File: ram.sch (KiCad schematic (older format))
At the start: 7 parts, among them U1 LFE5U-85F-6BG381C

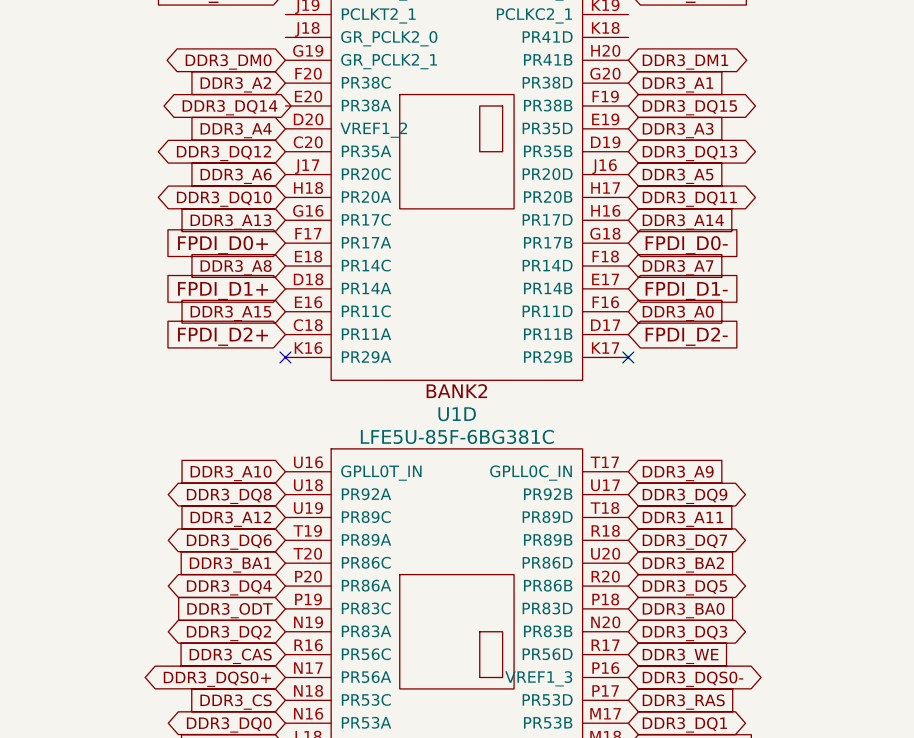
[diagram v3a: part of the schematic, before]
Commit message: More DDR3 routing
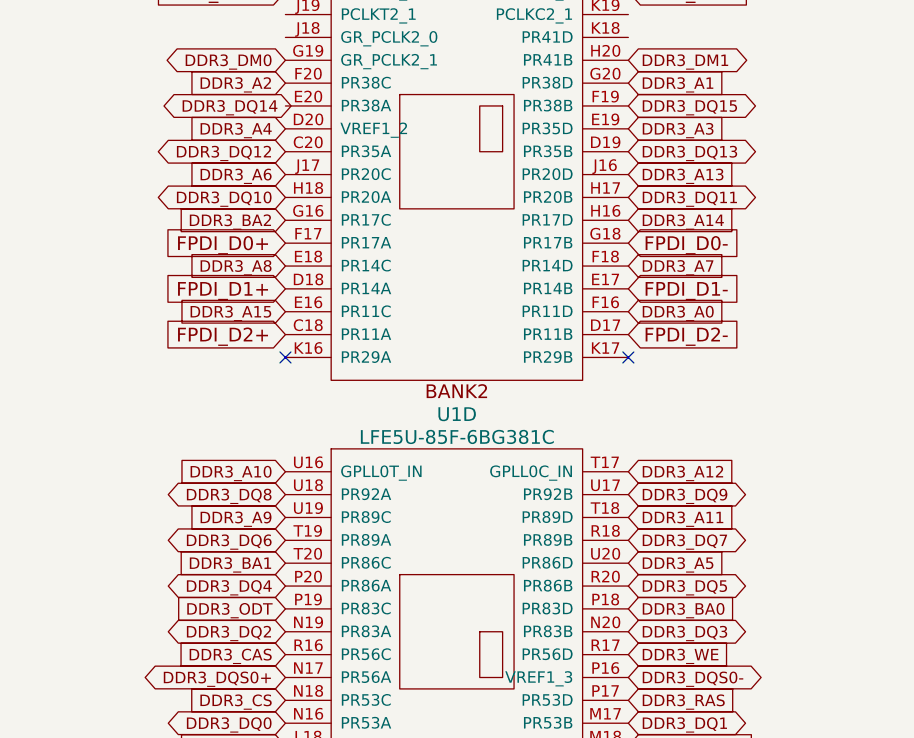
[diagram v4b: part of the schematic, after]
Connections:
- net DDR3_A12: now also U1.T17 (GPLL0C_IN); no longer U1.U19 (PR89C)
- net DDR3_A13: now also U1.J16 (PR20D); no longer U1.G16 (PR17C)
- net DDR3_A5: now also U1.U20 (PR86D); no longer U1.J16 (PR20D)
- net DDR3_A9: now also U1.U19 (PR89C); no longer U1.T17 (GPLL0C_IN)
- net DDR3_BA2: now also U1.G16 (PR17C); no longer U1.U20 (PR86D)
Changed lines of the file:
@@
 Text GLabel 6600 2300 0    50   Input ~ 0
 DDR3_A4
-Text GLabel 8100 2500 2    50   Input ~ 0
+Text GLabel 8100 4200 2    50   Input ~ 0
 DDR3_A5
 Text GLabel 6600 2500 0    50   Input ~ 0
@@
 Text GLabel 6600 2900 0    50   Input ~ 0
 DDR3_A8
-Text GLabel 8100 3800 2    50   Input ~ 0
+Text GLabel 6600 4000 0    50   Input ~ 0
 DDR3_A9
 Text GLabel 6600 3800 0    50   Input ~ 0
@@
 Text GLabel 8100 4000 2    50   Input ~ 0
 DDR3_A11
-Text GLabel 6600 4000 0    50   Input ~ 0
+Text GLabel 8100 3800 2    50   Input ~ 0
 DDR3_A12
-Text GLabel 6600 2700 0    50   Input ~ 0
+Text GLabel 8100 2500 2    50   Input ~ 0
 DDR3_A13
 Text GLabel 8100 2700 2    50   Input ~ 0
@@
 Text GLabel 6600 4200 0    50   Input ~ 0
 DDR3_BA1
-Text GLabel 8100 4200 2    50   Input ~ 0
+Text GLabel 6600 2700 0    50   Input ~ 0
 DDR3_BA2
 Text GLabel 6600 5300 0    50   Input ~ 0

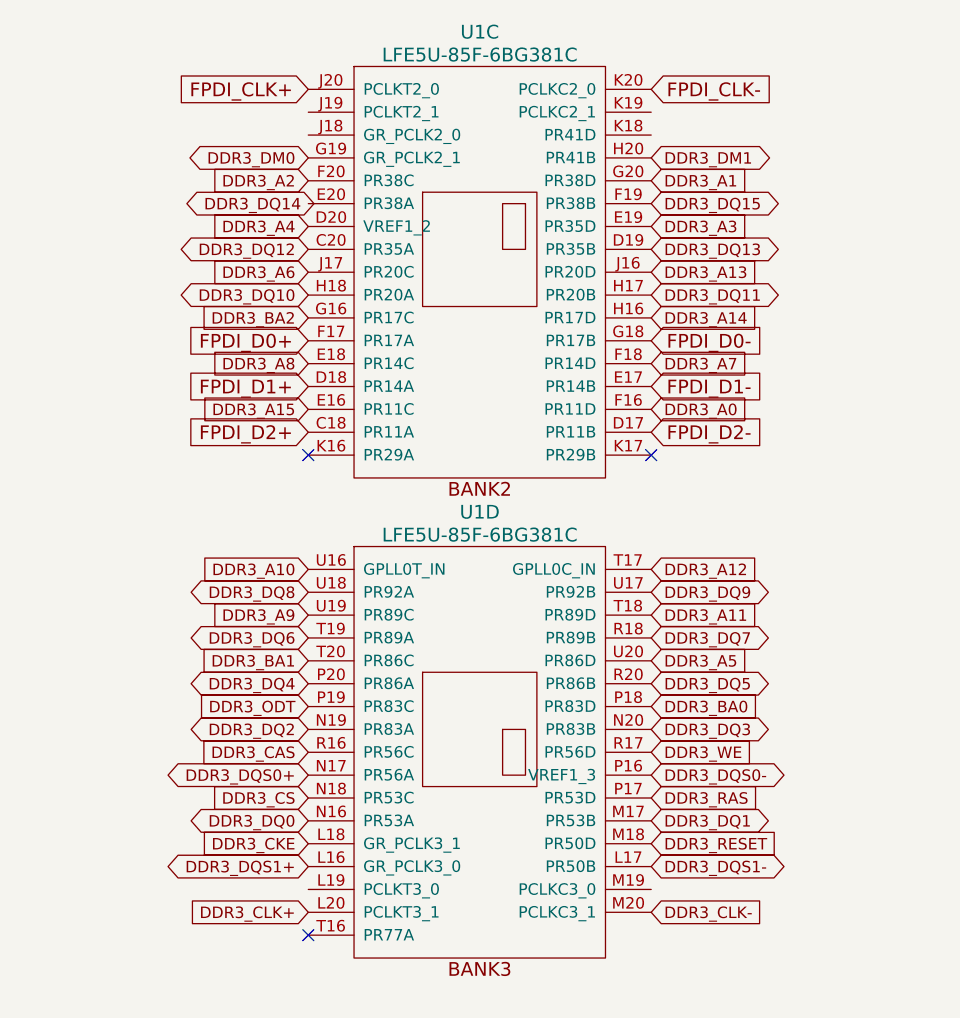
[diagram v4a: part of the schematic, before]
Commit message: Initial DDR3 signals routing
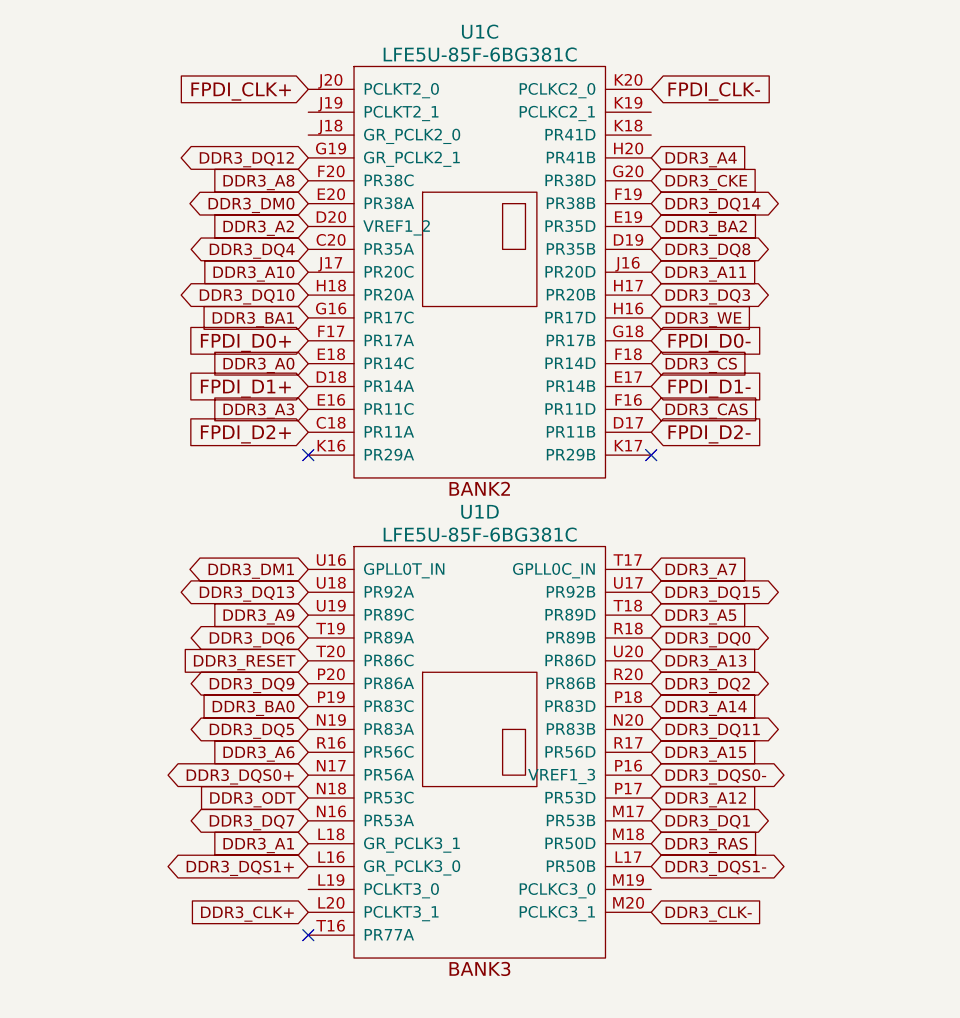
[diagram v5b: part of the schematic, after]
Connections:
- net DDR3_A0: now also U1.E18 (PR14C); no longer U1.F16 (PR11D)
- net DDR3_A1: now also U1.L18 (GR_PCLK3_1); no longer U1.G20 (PR38D)
- net DDR3_A10: now also U1.J17 (PR20C); no longer U1.U16 (GPLL0T_IN)
- net DDR3_A11: now also U1.J16 (PR20D); no longer U1.T18 (PR89D)
- net DDR3_A12: now also U1.P17 (PR53D); no longer U1.T17 (GPLL0C_IN)
- net DDR3_A13: now also U1.U20 (PR86D); no longer U1.J16 (PR20D)
- net DDR3_A14: now also U1.P18 (PR83D); no longer U1.H16 (PR17D)
- net DDR3_A15: now also U1.R17 (PR56D); no longer U1.E16 (PR11C)
- net DDR3_A2: now also U1.D20 (VREF1_2); no longer U1.F20 (PR38C)
- net DDR3_A3: now also U1.E16 (PR11C); no longer U1.E19 (PR35D)
- net DDR3_A4: now also U1.H20 (PR41B); no longer U1.D20 (VREF1_2)
- net DDR3_A5: now also U1.T18 (PR89D); no longer U1.U20 (PR86D)
- net DDR3_A6: now also U1.R16 (PR56C); no longer U1.J17 (PR20C)
- net DDR3_A7: now also U1.T17 (GPLL0C_IN); no longer U1.F18 (PR14D)
- net DDR3_A8: now also U1.F20 (PR38C); no longer U1.E18 (PR14C)
- net DDR3_BA0: now also U1.P19 (PR83C); no longer U1.P18 (PR83D)
- net DDR3_BA1: now also U1.G16 (PR17C); no longer U1.T20 (PR86C)
- net DDR3_BA2: now also U1.E19 (PR35D); no longer U1.G16 (PR17C)
- net DDR3_CAS: now also U1.F16 (PR11D); no longer U1.R16 (PR56C)
- net DDR3_CKE: now also U1.G20 (PR38D); no longer U1.L18 (GR_PCLK3_1)
- net DDR3_CS: now also U1.F18 (PR14D); no longer U1.N18 (PR53C)
- net DDR3_DM0: now also U1.E20 (PR38A); no longer U1.G19 (GR_PCLK2_1)
- net DDR3_DM1: now also U1.U16 (GPLL0T_IN); no longer U1.H20 (PR41B)
- net DDR3_DQ0: now also U1.R18 (PR89B); no longer U1.N16 (PR53A)
- net DDR3_DQ11: now also U1.N20 (PR83B); no longer U1.H17 (PR20B)
- net DDR3_DQ12: now also U1.G19 (GR_PCLK2_1); no longer U1.C20 (PR35A)
- net DDR3_DQ13: now also U1.U18 (PR92A); no longer U1.D19 (PR35B)
- net DDR3_DQ14: now also U1.F19 (PR38B)
- net DDR3_DQ15: now also U1.U17 (PR92B); no longer U1.F19 (PR38B)
- net DDR3_DQ2: now also U1.R20 (PR86B); no longer U1.N19 (PR83A)
- net DDR3_DQ3: now also U1.H17 (PR20B); no longer U1.N20 (PR83B)
- net DDR3_DQ4: now also U1.C20 (PR35A); no longer U1.P20 (PR86A)
- net DDR3_DQ5: now also U1.N19 (PR83A); no longer U1.R20 (PR86B)
- net DDR3_DQ7: now also U1.N16 (PR53A); no longer U1.R18 (PR89B)
- net DDR3_DQ8: now also U1.D19 (PR35B); no longer U1.U18 (PR92A)
- net DDR3_DQ9: now also U1.P20 (PR86A); no longer U1.U17 (PR92B)
- net DDR3_ODT: now also U1.N18 (PR53C); no longer U1.P19 (PR83C)
- net DDR3_RAS: now also U1.M18 (PR50D); no longer U1.P17 (PR53D)
- net DDR3_RESET: now also U1.T20 (PR86C); no longer U1.M18 (PR50D)
- net DDR3_WE: now also U1.H16 (PR17D); no longer U1.R17 (PR56D)
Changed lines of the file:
@@
 Text GLabel 1475 7250 0    60   Input ~ 0
 SD_D2
-Text GLabel 8100 3100 2    50   Input ~ 0
+Text GLabel 6600 2900 0    50   Input ~ 0
 DDR3_A0
-Text GLabel 8100 2100 2    50   Input ~ 0
+Text GLabel 6600 5000 0    50   Input ~ 0
 DDR3_A1
+Text GLabel 6600 2300 0    50   Input ~ 0
+DDR3_A2
+Text GLabel 6600 3100 0    50   Input ~ 0
+DDR3_A3
+Text GLabel 8100 2000 2    50   Input ~ 0
+DDR3_A4
+Text GLabel 6600 4600 0    50   Input ~ 0
+DDR3_A6
+Text GLabel 8100 3800 2    50   Input ~ 0
+DDR3_A7
 Text GLabel 6600 2100 0    50   Input ~ 0
-DDR3_A2
-Text GLabel 8100 2300 2    50   Input ~ 0
-DDR3_A3
-Text GLabel 6600 2300 0    50   Input ~ 0
-DDR3_A4
-Text GLabel 8100 4200 2    50   Input ~ 0
-DDR3_A5
-Text GLabel 6600 2500 0    50   Input ~ 0
-DDR3_A6
-Text GLabel 8100 2900 2    50   Input ~ 0
-DDR3_A7
-Text GLabel 6600 2900 0    50   Input ~ 0
 DDR3_A8
 Text GLabel 6600 4000 0    50   Input ~ 0
 DDR3_A9
-Text GLabel 6600 3800 0    50   Input ~ 0
+Text GLabel 6600 2500 0    50   Input ~ 0
 DDR3_A10
-Text GLabel 8100 4000 2    50   Input ~ 0
+Text GLabel 8100 2500 2    50   Input ~ 0
 DDR3_A11
-Text GLabel 8100 3800 2    50   Input ~ 0
+Text GLabel 8100 4800 2    50   Input ~ 0
 DDR3_A12
-Text GLabel 8100 2500 2    50   Input ~ 0
-DDR3_A13
-Text GLabel 8100 2700 2    50   Input ~ 0
+Text GLabel 8100 4400 2    50   Input ~ 0
 DDR3_A14
-Text GLabel 8100 4400 2    50   Input ~ 0
+Text GLabel 6600 4400 0    50   Input ~ 0
 DDR3_BA0
-Text GLabel 6600 4200 0    50   Input ~ 0
+Text GLabel 6600 2700 0    50   Input ~ 0
 DDR3_BA1
-Text GLabel 6600 2700 0    50   Input ~ 0
+Text GLabel 8100 2300 2    50   Input ~ 0
 DDR3_BA2
 Text GLabel 6600 5300 0    50   Input ~ 0
@@
 Text GLabel 8100 5300 2    50   Input ~ 0
 DDR3_CLK-
-Text GLabel 6600 5000 0    50   Input ~ 0
+Text GLabel 8100 2100 2    50   Input ~ 0
 DDR3_CKE
+Text GLabel 6600 4200 0    50   Input ~ 0
+DDR3_RESET
+Text GLabel 8100 2900 2    50   Input ~ 0
+DDR3_CS
+Text GLabel 8100 3100 2    50   Input ~ 0
+DDR3_CAS
 Text GLabel 8100 5000 2    50   Input ~ 0
-DDR3_RESET
+DDR3_RAS
+Text GLabel 8100 2700 2    50   Input ~ 0
+DDR3_WE
 Text GLabel 6600 4800 0    50   Input ~ 0
-DDR3_CS
-Text GLabel 6600 4600 0    50   Input ~ 0
-DDR3_CAS
-Text GLabel 8100 4800 2    50   Input ~ 0
-DDR3_RAS
-Text GLabel 8100 4600 2    50   Input ~ 0
-DDR3_WE
-Text GLabel 6600 4400 0    50   Input ~ 0
 DDR3_ODT
-Text GLabel 6600 4900 0    50   BiDi ~ 0
+Text GLabel 8100 4100 2    50   BiDi ~ 0
 DDR3_DQ0
 Text GLabel 8100 4900 2    50   BiDi ~ 0
 DDR3_DQ1
+Text GLabel 8100 4300 2    50   BiDi ~ 0
+DDR3_DQ2
+Text GLabel 8100 2600 2    50   BiDi ~ 0
+DDR3_DQ3
+Text GLabel 6600 2400 0    50   BiDi ~ 0
+DDR3_DQ4
 Text GLabel 6600 4500 0    50   BiDi ~ 0
-DDR3_DQ2
-Text GLabel 8100 4500 2    50   BiDi ~ 0
-DDR3_DQ3
-Text GLabel 6600 4300 0    50   BiDi ~ 0
-DDR3_DQ4
-Text GLabel 8100 4300 2    50   BiDi ~ 0
 DDR3_DQ5
 Text GLabel 6600 4100 0    50   BiDi ~ 0
 DDR3_DQ6
-Text GLabel 8100 4100 2    50   BiDi ~ 0
+Text GLabel 6600 4900 0    50   BiDi ~ 0
 DDR3_DQ7
-Text GLabel 6600 3900 0    50   BiDi ~ 0
+Text GLabel 8100 2400 2    50   BiDi ~ 0
 DDR3_DQ8
-Text GLabel 8100 3900 2    50   BiDi ~ 0
-DDR3_DQ9
 Text GLabel 6600 2600 0    50   BiDi ~ 0
 DDR3_DQ10
-Text GLabel 8100 2600 2    50   BiDi ~ 0
+Text GLabel 8100 4500 2    50   BiDi ~ 0
 DDR3_DQ11
-Text GLabel 6600 2400 0    50   BiDi ~ 0
+Text GLabel 6600 2000 0    50   BiDi ~ 0
 DDR3_DQ12
-Text GLabel 8100 2400 2    50   BiDi ~ 0
-DDR3_DQ13
-Text GLabel 6625 2200 0    50   BiDi ~ 0
+Text GLabel 8100 2200 2    50   BiDi ~ 0
 DDR3_DQ14
-Text GLabel 8100 2200 2    50   BiDi ~ 0
+Text GLabel 8100 3900 2    50   BiDi ~ 0
 DDR3_DQ15
-Text GLabel 6600 2000 0    50   BiDi ~ 0
-DDR3_DM0
-Text GLabel 8100 2000 2    50   BiDi ~ 0
+Text GLabel 6600 3800 0    50   BiDi ~ 0
 DDR3_DM1
 Text GLabel 6600 4700 0    50   BiDi ~ 0
@@
 Text GLabel 2125 7000 0    60   Input ~ 0
 GPIO10
-Text GLabel 6600 3100 0    50   Input ~ 0
+Text GLabel 8100 4600 2    50   Input ~ 0
 DDR3_A15
+Text GLabel 8100 4000 2    50   Input ~ 0
+DDR3_A5
+Text GLabel 8100 4200 2    50   Input ~ 0
+DDR3_A13
+Text GLabel 6600 4300 0    50   BiDi ~ 0
+DDR3_DQ9
+Text GLabel 6600 3900 0    50   BiDi ~ 0
+DDR3_DQ13
+Text GLabel 6600 2200 0    50   BiDi ~ 0
+DDR3_DM0
 $EndSCHEMATC

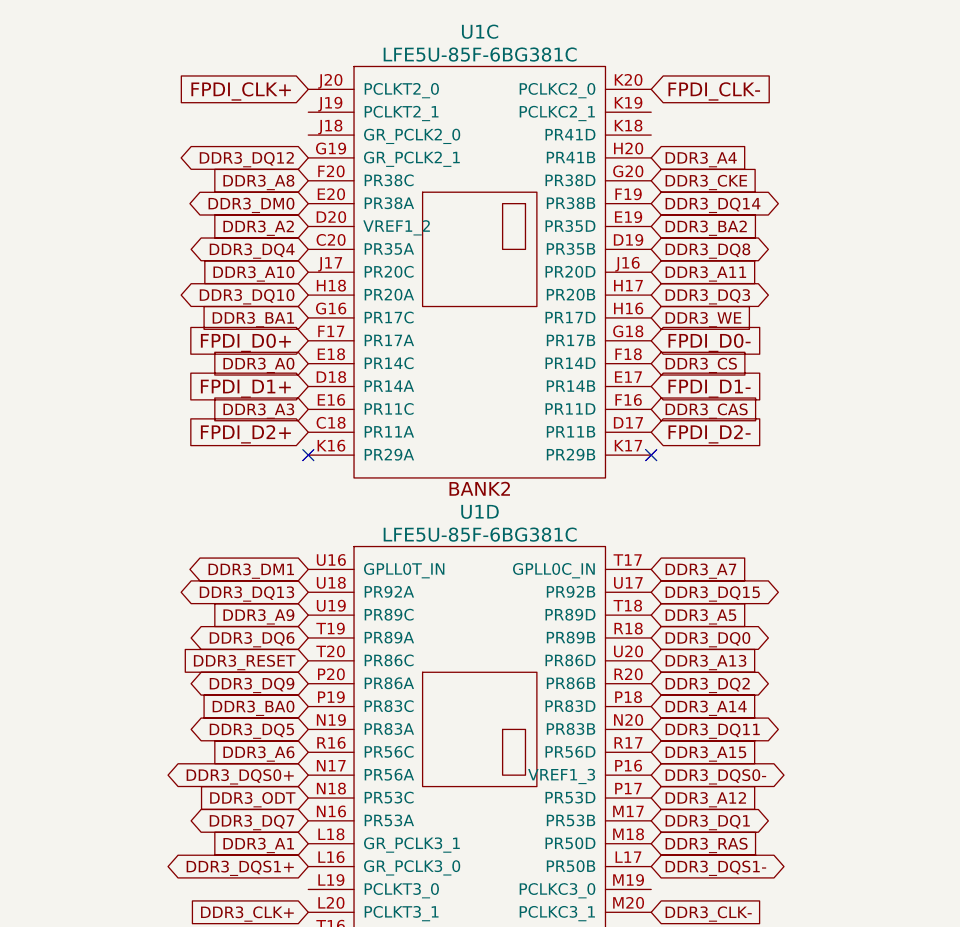
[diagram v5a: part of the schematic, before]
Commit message: Improved routing
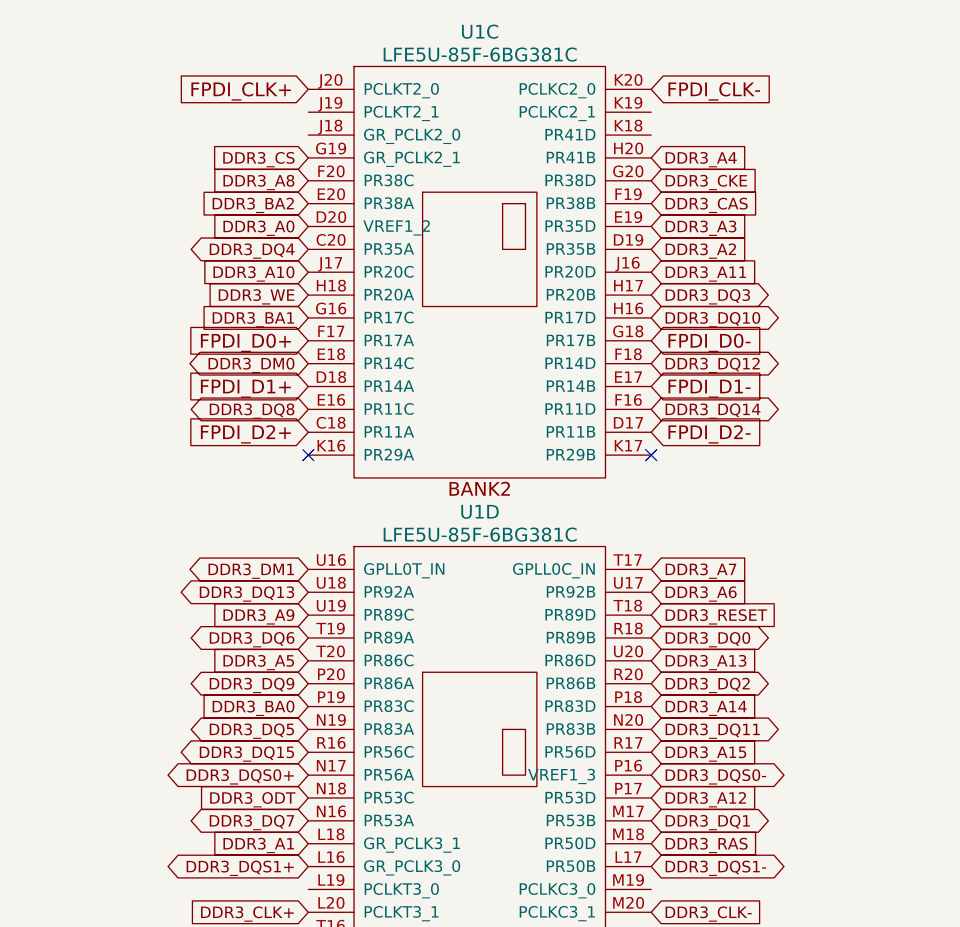
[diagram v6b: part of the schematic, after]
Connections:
- net DDR3_A0: now also U1.D20 (VREF1_2); no longer U1.E18 (PR14C)
- net DDR3_A2: now also U1.D19 (PR35B); no longer U1.D20 (VREF1_2)
- net DDR3_A3: now also U1.E19 (PR35D); no longer U1.E16 (PR11C)
- net DDR3_A5: now also U1.T20 (PR86C); no longer U1.T18 (PR89D)
- net DDR3_A6: now also U1.U17 (PR92B); no longer U1.R16 (PR56C)
- net DDR3_BA2: now also U1.E20 (PR38A); no longer U1.E19 (PR35D)
- net DDR3_CAS: now also U1.F19 (PR38B); no longer U1.F16 (PR11D)
- net DDR3_CS: now also U1.G19 (GR_PCLK2_1); no longer U1.F18 (PR14D)
- net DDR3_DM0: now also U1.E18 (PR14C); no longer U1.E20 (PR38A)
- net DDR3_DQ10: now also U1.H16 (PR17D); no longer U1.H18 (PR20A)
- net DDR3_DQ12: now also U1.F18 (PR14D); no longer U1.G19 (GR_PCLK2_1)
- net DDR3_DQ14: now also U1.F16 (PR11D); no longer U1.F19 (PR38B)
- net DDR3_DQ15: now also U1.R16 (PR56C); no longer U1.U17 (PR92B)
- net DDR3_DQ8: now also U1.E16 (PR11C); no longer U1.D19 (PR35B)
- net DDR3_RESET: now also U1.T18 (PR89D); no longer U1.T20 (PR86C)
- net DDR3_WE: now also U1.H18 (PR20A); no longer U1.H16 (PR17D)
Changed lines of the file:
@@
 Text GLabel 1475 7250 0    60   Input ~ 0
 SD_D2
-Text GLabel 6600 2900 0    50   Input ~ 0
+Text GLabel 6600 2300 0    50   Input ~ 0
 DDR3_A0
 Text GLabel 6600 5000 0    50   Input ~ 0
 DDR3_A1
-Text GLabel 6600 2300 0    50   Input ~ 0
+Text GLabel 8100 2400 2    50   Input ~ 0
 DDR3_A2
-Text GLabel 6600 3100 0    50   Input ~ 0
+Text GLabel 8100 2300 2    50   Input ~ 0
 DDR3_A3
 Text GLabel 8100 2000 2    50   Input ~ 0
 DDR3_A4
-Text GLabel 6600 4600 0    50   Input ~ 0
+Text GLabel 8100 3900 2    50   Input ~ 0
 DDR3_A6
 Text GLabel 8100 3800 2    50   Input ~ 0
@@
 Text GLabel 6600 2700 0    50   Input ~ 0
 DDR3_BA1
-Text GLabel 8100 2300 2    50   Input ~ 0
+Text GLabel 6600 2200 0    50   Input ~ 0
 DDR3_BA2
 Text GLabel 6600 5300 0    50   Input ~ 0
@@
 Text GLabel 8100 2100 2    50   Input ~ 0
 DDR3_CKE
-Text GLabel 6600 4200 0    50   Input ~ 0
+Text GLabel 8100 4000 2    50   Input ~ 0
 DDR3_RESET
-Text GLabel 8100 2900 2    50   Input ~ 0
+Text GLabel 6600 2000 0    50   Input ~ 0
 DDR3_CS
-Text GLabel 8100 3100 2    50   Input ~ 0
+Text GLabel 8100 2200 2    50   Input ~ 0
 DDR3_CAS
 Text GLabel 8100 5000 2    50   Input ~ 0
 DDR3_RAS
-Text GLabel 8100 2700 2    50   Input ~ 0
+Text GLabel 6600 2600 0    50   Input ~ 0
 DDR3_WE
 Text GLabel 6600 4800 0    50   Input ~ 0
@@
 Text GLabel 6600 4900 0    50   BiDi ~ 0
 DDR3_DQ7
-Text GLabel 8100 2400 2    50   BiDi ~ 0
+Text GLabel 6600 3100 0    50   BiDi ~ 0
 DDR3_DQ8
-Text GLabel 6600 2600 0    50   BiDi ~ 0
+Text GLabel 8100 2700 2    50   BiDi ~ 0
 DDR3_DQ10
 Text GLabel 8100 4500 2    50   BiDi ~ 0
 DDR3_DQ11
-Text GLabel 6600 2000 0    50   BiDi ~ 0
+Text GLabel 8100 2900 2    50   BiDi ~ 0
 DDR3_DQ12
-Text GLabel 8100 2200 2    50   BiDi ~ 0
+Text GLabel 8100 3100 2    50   BiDi ~ 0
 DDR3_DQ14
-Text GLabel 8100 3900 2    50   BiDi ~ 0
+Text GLabel 6600 4600 0    50   BiDi ~ 0
 DDR3_DQ15
 Text GLabel 6600 3800 0    50   BiDi ~ 0
@@
 Text GLabel 8100 4600 2    50   Input ~ 0
 DDR3_A15
-Text GLabel 8100 4000 2    50   Input ~ 0
+Text GLabel 6600 4200 0    50   Input ~ 0
 DDR3_A5
 Text GLabel 8100 4200 2    50   Input ~ 0
@@
 Text GLabel 6600 3900 0    50   BiDi ~ 0
 DDR3_DQ13
-Text GLabel 6600 2200 0    50   BiDi ~ 0
+Text GLabel 6600 2900 0    50   BiDi ~ 0
 DDR3_DM0
 $EndSCHEMATC
